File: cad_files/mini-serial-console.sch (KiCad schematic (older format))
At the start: 37 parts, among them J1 Screw_Terminal_1x02, J2 Screw_Terminal_1x03, J3 DB9M, J4 Screw_Terminal_1x05, P1 10k, Q1 BC559, Q2 BC548, U1 HD44780 compatible LCD, U2 Pico

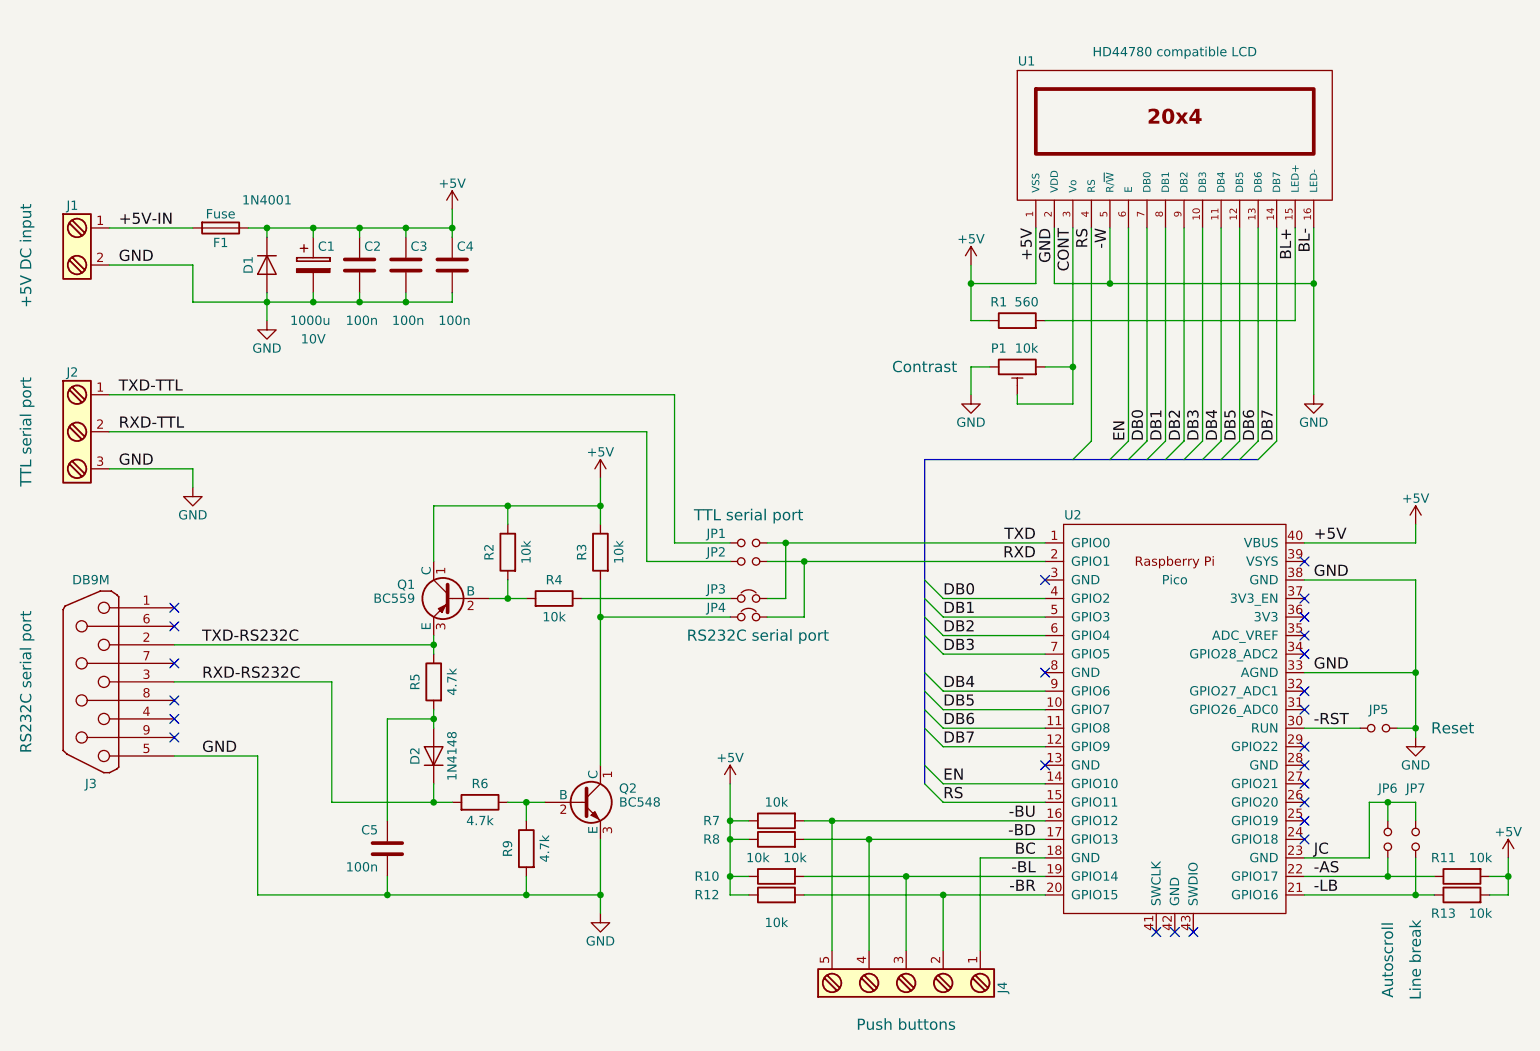
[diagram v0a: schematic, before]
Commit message: 220930
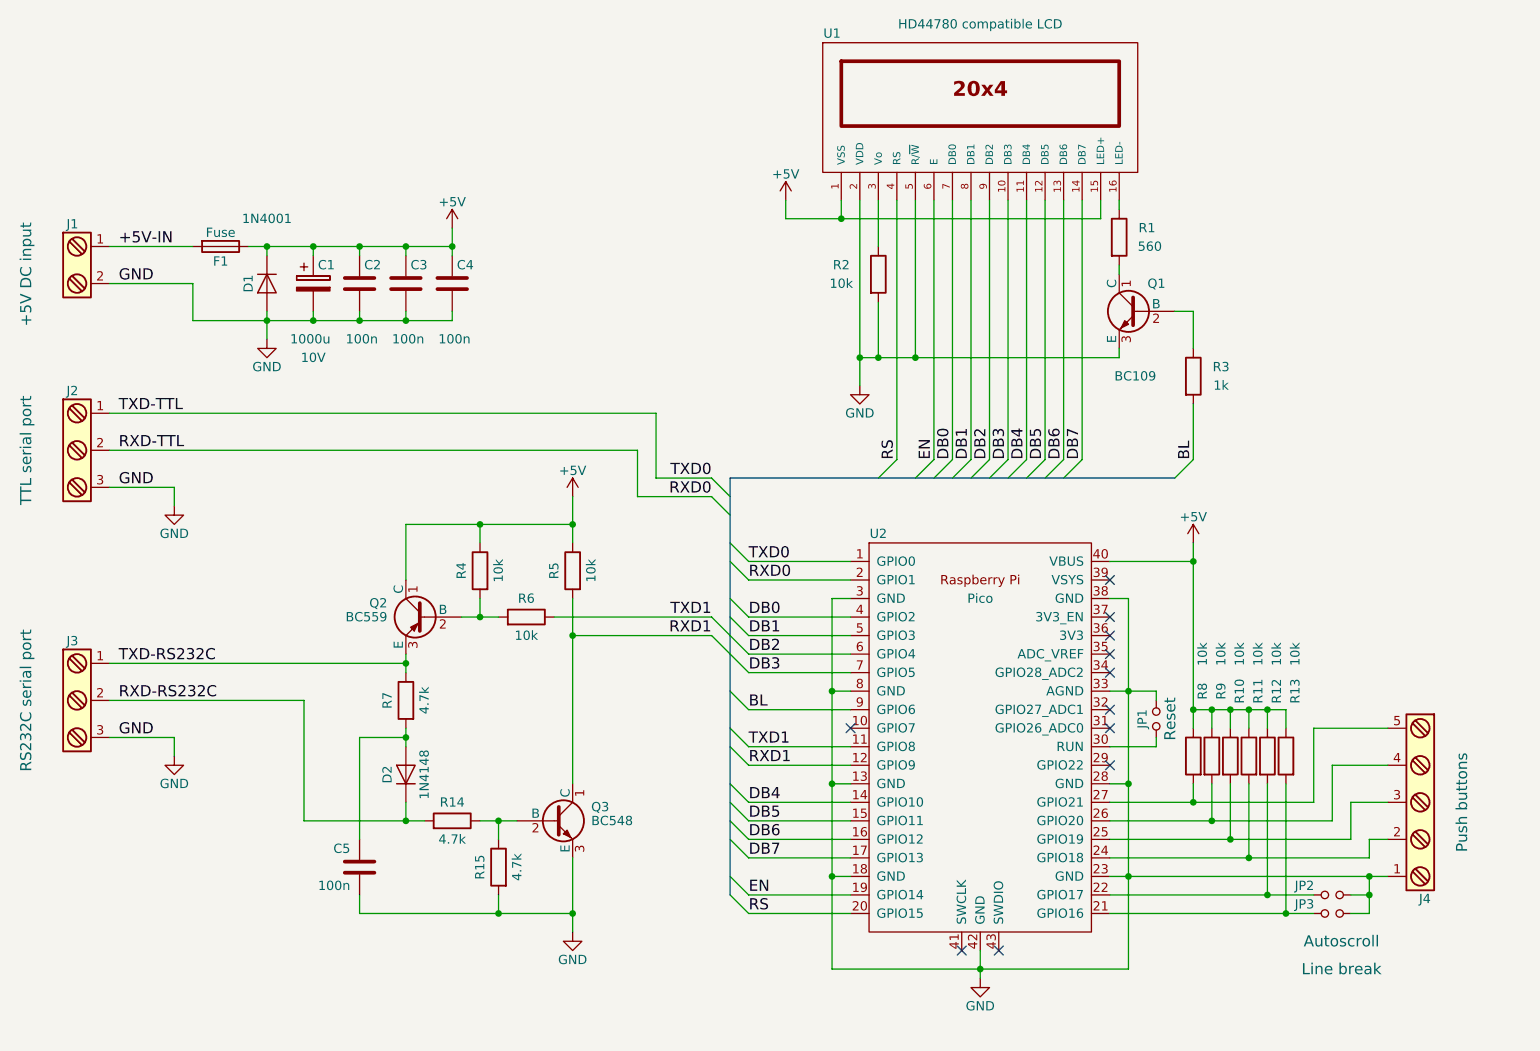
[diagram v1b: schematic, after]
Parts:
- removed J3: DB9M, Connectors:DB9MC, symbol DB9
- removed JP1, JP2: Jumper_NO_Small, Socket_Strips:Socket_Strip_Straight_1x02, symbol Jumper_NO_Small
- removed JP3, JP4: Jumper_NC_Small, Socket_Strips:Socket_Strip_Straight_1x02, symbol Jumper_NC_Small
- removed P1: 10k, Potentiometers:Potentiometer_WirePads_Small, symbol POT_TRIM
- added J3: Screw_Terminal_1x03, Connectors:bornier3, symbol Screw_Terminal_1x03
- added Q1: BC109, TO_SOT_Packages_THT:TO-18-3, symbol BC548
- added R2: 10k, Resistors_THT:R_Axial_DIN0411_L9.9mm_D3.6mm_P12.70mm_Horizontal, symbol R
- added R3: 1k, Resistors_THT:R_Axial_DIN0411_L9.9mm_D3.6mm_P12.70mm_Horizontal, symbol R
- renumbered JP5 to JP1, JP6 to JP2, JP7 to JP3, Q1 to Q2, Q2 to Q3, R7 to R10, R8 to R11, R10 to R12, R12 to R13, R6 to R14, R9 to R15, R2 to R4, R3 to R5, R4 to R6, R5 to R7, R13 to R8, R11 to R9
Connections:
- net BC is gone; now on net GND: J4.1, U2.18 (GND)
- net RXD is gone; now on net RXD-TTL: U2.2 (GPIO1)
- net TXD is gone; now on net TXD-TTL: U2.1 (GPIO0)
- net +5V: now also R8.1, R9.1, U1.15 (LED+); no longer R1.1, R8.2, R9.2
- net DB4: now also U2.14 (GPIO10); no longer U2.9 (GPIO6)
- net DB5: now also U2.15 (GPIO11); no longer U2.10 (GPIO7)
- net DB6: now also U2.16 (GPIO12); no longer U2.11 (GPIO8)
- net DB7: now also U2.17 (GPIO13); no longer U2.12 (GPIO9)
- net EN: now also U2.19 (GPIO14); no longer U2.14 (GPIO10)
- net GND: now also JP2.2, JP3.2, U2.13 (GND), U2.23 (GND), U2.28 (GND), U2.3 (GND), U2.42 (GND), U2.8 (GND), J3.3, Q1.3 (E), R2.2; no longer U1.16 (LED-)
- net RS: now also U2.20 (GPIO15); no longer U2.15 (GPIO11)
- net RXD-RS232C: now also J3.2
- net TXD-RS232C: now also J3.1
- net RXD1: now reaches Q3.1 (C), R5.2
- net RXD1: now also U2.12 (GPIO9)
- net TXD1: now reaches R6.1
- net TXD1: now also U2.11 (GPIO8)
- net at U2.24 (GPIO18): now also J4.2, R11.2
- net at U2.25 (GPIO19): now also J4.3, R10.2
- net at U2.26 (GPIO20): now also J4.4, R8.2
- net at U2.27 (GPIO21): now also J4.5, R9.2
- removed net -AS: JP2.2, R9.1, U2.22 (GPIO17)
- removed net -BD: J4.4, R11.2, U2.17 (GPIO13)
- removed net -BL: J4.3, R12.2, U2.19 (GPIO14)
- removed net -BR: J4.2, R13.2, U2.20 (GPIO15)
- removed net -BU: J4.5, R10.2, U2.16 (GPIO12)
- removed net -LB: JP3.2, R8.1, U2.21 (GPIO16)
- net -RST: no longer names the net of JP1.1, U2.30 (RUN)
- net BL+: no longer names the net of R1.2
- net BL+: now also Q1.1 (C); no longer U1.15 (LED+)
- net CONT: no longer names the net of U1.3 (Vo)
- net CONT: now also R2.1
- removed net JC: JP2.1, JP3.1, U2.23 (GND)
- new net: R1.1, U1.16 (LED-)
- new net: JP3.1, R13.2, U2.21 (GPIO16)
- new net: JP2.1, R12.2, U2.22 (GPIO17)
- new net: Q1.2 (B), R3.1
- new net BL: R3.2, U2.9 (GPIO6)
- no-connect marks 25 -> 11
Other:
- moved on the sheet: C1, C2, C3, C4, C5, D1, D2, F1, J1, J2, J4, JP1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
